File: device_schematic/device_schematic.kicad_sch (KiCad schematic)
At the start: 1 part

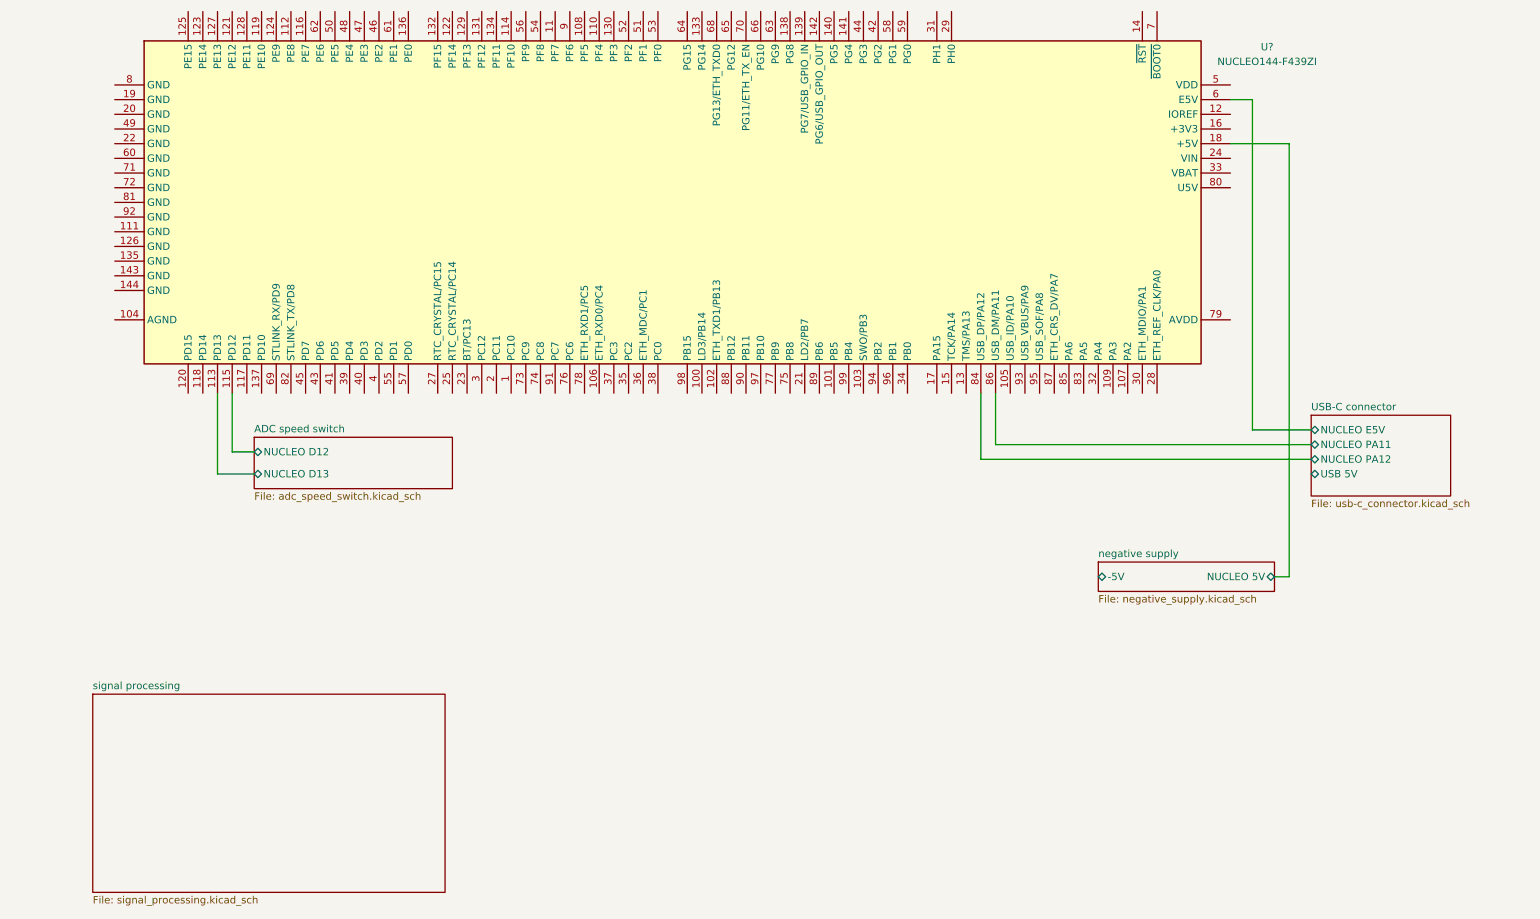
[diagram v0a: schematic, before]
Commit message: Device schematic update
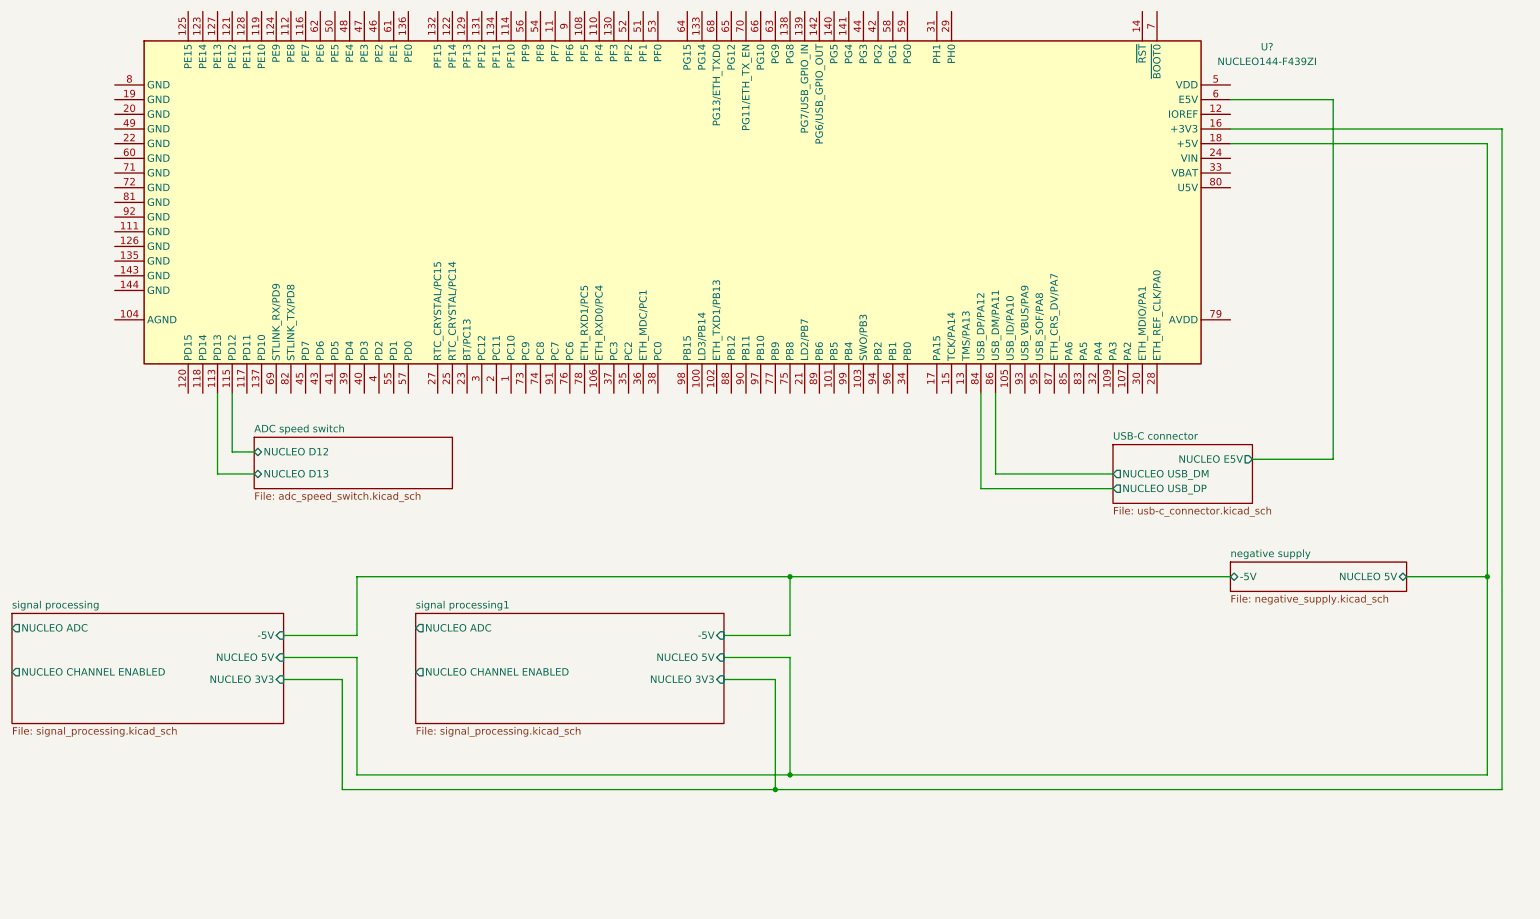
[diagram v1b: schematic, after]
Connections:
- net signal processing/NUCLEO 3V3: now reaches U?.16 (+3V3)
- net USB-C connector/NUCLEO PA11 renamed USB-C connector/NUCLEO USB_DM
- net USB-C connector/NUCLEO PA12 renamed USB-C connector/NUCLEO USB_DP
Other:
- added sheet signal processing1 (signal_processing.kicad_sch)
- sheet USB-C connector ports: added NUCLEO USB_DM, NUCLEO USB_DP; removed NUCLEO PA11, NUCLEO PA12, USB 5V
- sheet signal processing ports: added -5V, NUCLEO 3V3, NUCLEO 5V, NUCLEO ADC, NUCLEO CHANNEL ENABLED; removed none
